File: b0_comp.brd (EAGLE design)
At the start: 93 x 70 mm, 287 parts, among them IC1 КР1006ВИ1(NE555), IC3 LM358D, IC4 78L09F, IC5 XL6009S, IC6 MEGA8-AI, IC7 74121N, IC8 4030N, IC9 LM324D, T1P T90, -26 MicroMetals Yellow-W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

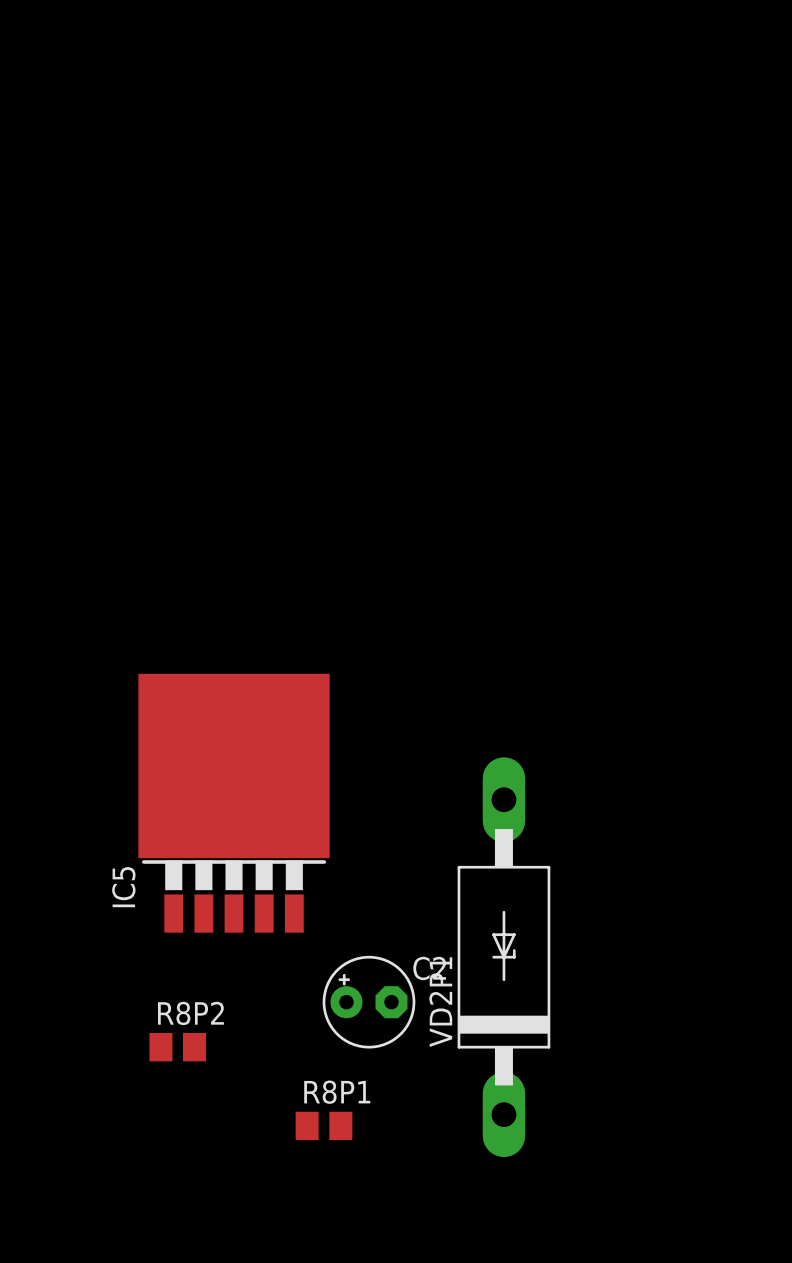
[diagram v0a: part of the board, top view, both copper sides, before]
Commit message: .
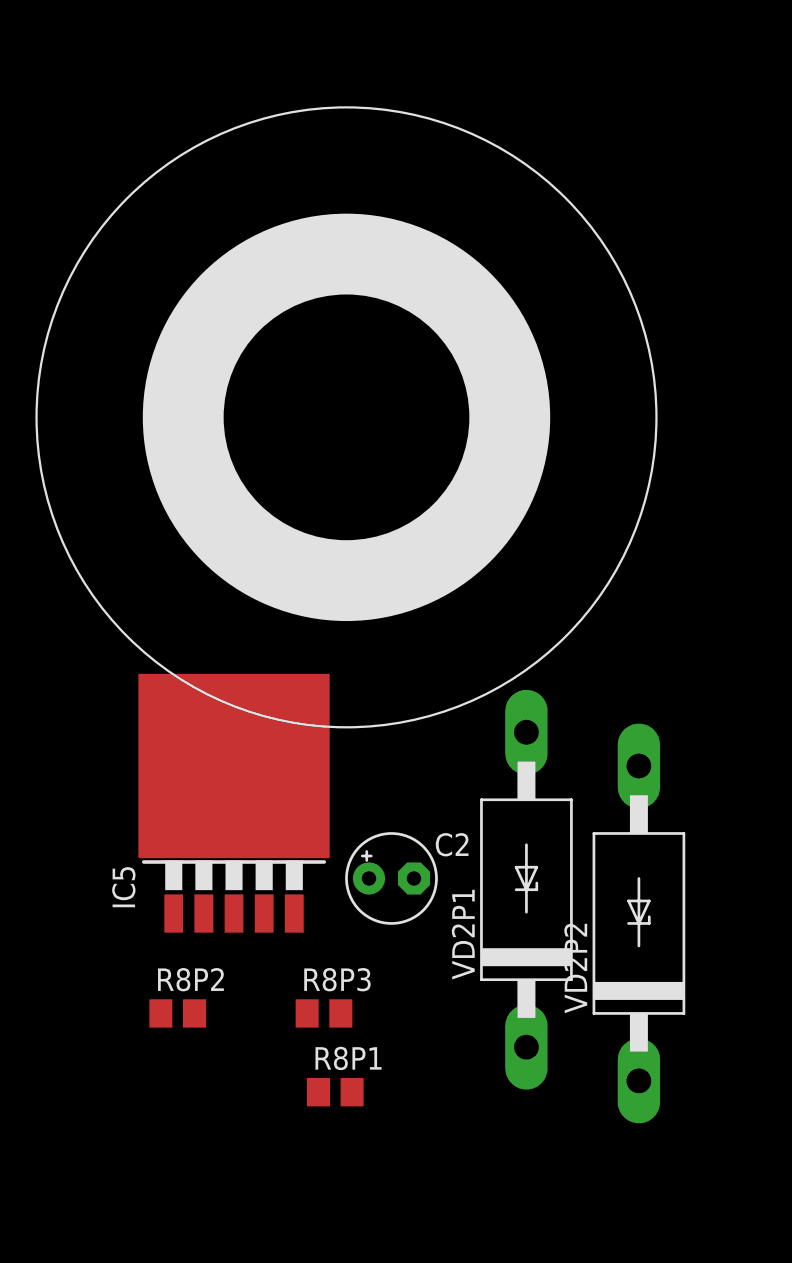
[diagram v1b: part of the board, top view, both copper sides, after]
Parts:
- added R8P3: 3k, rcl:M0805
- added T1P1: T90, -26 MicroMetals Yellow-White, b0f:R23X14
- added VD2P2: SR5200, diode:CB429-17
- C2: value (none) -> 22m
- IC5: value XL6009S -> XL6009
- moved C2 7.10 mm to (-367.7, 91.4)
- moved VD2P1 4.02 mm to (-360.0, 90.8)
- moved R8P1 2.01 mm to (-370.8, 79.4)
- moved R8P2 1.90 mm to (-379.7, 83.8)
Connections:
- new net N$190: C2.-, VD2P2.A
- new net N$191: VD2P2.C
- net N$187: now also R8P3.2; no longer R8P1.2
- net N$188: no longer C2.-
- net N$189: now also R8P3.1; no longer R8P1.1
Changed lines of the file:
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@@
 <element name="R22" library="rcl" package="M0805" value="27" x="-275.59" y="114.3" rot="MR180"/>
 <element name="R23" library="rcl" package="M0805" value="27" x="-276.225" y="123.19" rot="MR180"/>
-<element name="IC5" library="XL6009" package="TO263-5" value="XL6009S" x="-376.555" y="95.25"/>
-<element name="VD2P1" library="diode" package="CB429-17" value="SR5200" x="-361.315" y="86.995" rot="R90"/>
-<element name="C2" library="rcl" package="E2,5-5" value="" x="-368.935" y="84.455"/>
-<element name="R8P1" library="rcl" package="M0805" value="8k6" x="-371.475" y="77.47"/>
-<element name="R8P2" library="rcl" package="M0805" value="1k" x="-379.73" y="81.915"/>
+<element name="IC5" library="XL6009" package="TO263-5" value="XL6009" x="-376.555" y="95.25"/>
+<element name="VD2P1" library="diode" package="CB429-17" value="SR5200" x="-360.045" y="90.805" rot="R90"/>
+<element name="C2" library="rcl" package="E2,5-5" value="22m" x="-367.665" y="91.44"/>
+<element name="R8P1" library="rcl" package="M0805" value="8k6" x="-370.84" y="79.375"/>
+<element name="R8P2" library="rcl" package="M0805" value="1k" x="-379.73" y="83.82"/>
+<element name="R8P3" library="rcl" package="M0805" value="3k" x="-371.475" y="83.82"/>
+<element name="T1P1" library="b0f" package="R23X14" value="T90, -26 MicroMetals Yellow-White" x="-370.205" y="117.475"/>
+<element name="VD2P2" library="diode" package="CB429-17" value="SR5200" x="-353.695" y="88.9" rot="R90"/>
 </elements>
 <signals>
@@
 <wire x1="-367.0275" y1="-35.2425" x2="-364.4265" y2="-29.5275" width="0" layer="19" extent="1-1"/>
 <wire x1="-364.4265" y1="-39.0525" x2="-367.0275" y2="-35.2425" width="0" layer="19" extent="1-1"/>
-<wire x1="-380.68" y1="81.915" x2="-367.3475" y2="-3.4925" width="0" layer="19" extent="1-1"/>
-<wire x1="-379.9586" y1="89.4588" x2="-380.68" y2="81.915" width="0" layer="19" extent="1-1"/>
+<wire x1="-380.68" y1="83.82" x2="-367.3475" y2="-3.4925" width="0" layer="19" extent="1-1"/>
+<wire x1="-379.9586" y1="89.4588" x2="-380.68" y2="83.82" width="0" layer="19" extent="1-1"/>
 <wire x1="-378.2568" y1="89.4588" x2="-379.9586" y2="89.4588" width="0" layer="19" extent="1-1"/>
 </signal>
@@
 <contactref element="IC5" pad="3"/>
 <contactref element="C2" pad="+"/>
-<wire x1="-370.205" y1="84.455" x2="-376.555" y2="89.4588" width="0" layer="19" extent="1-1"/>
+<wire x1="-368.935" y1="91.44" x2="-376.555" y2="89.4588" width="0" layer="19" extent="1-1"/>
 </signal>
 <signal name="N$186">
@@
 <signal name="N$188">
 <contactref element="VD2P1" pad="A"/>
-<contactref element="C2" pad="-"/>
-<wire x1="-361.315" y1="95.885" x2="-367.665" y2="84.455" width="0" layer="19" extent="1-1"/>
 </signal>
 <signal name="N$187">
 <contactref element="VD2P1" pad="C"/>
-<contactref element="R8P1" pad="2"/>
-<wire x1="-361.315" y1="78.105" x2="-370.525" y2="77.47" width="0" layer="19" extent="1-1"/>
+<contactref element="R8P3" pad="2"/>
+<wire x1="-370.525" y1="83.82" x2="-360.045" y2="81.915" width="0" layer="19" extent="1-1"/>
 </signal>
 <signal name="N$189">
-<contactref element="R8P1" pad="1"/>
 <contactref element="R8P2" pad="2"/>
 <contactref element="IC5" pad="5"/>
-<wire x1="-372.425" y1="77.47" x2="-378.78" y2="81.915" width="0" layer="19" extent="1-1"/>
-<wire x1="-373.1514" y1="89.4588" x2="-378.78" y2="81.915" width="0" layer="19" extent="1-1"/>
+<contactref element="R8P3" pad="1"/>
+<wire x1="-373.1514" y1="89.4588" x2="-378.78" y2="83.82" width="0" layer="19" extent="1-1"/>
+<wire x1="-372.425" y1="83.82" x2="-378.78" y2="83.82" width="0" layer="19" extent="1-1"/>
+</signal>
+<signal name="N$190">
+<contactref element="C2" pad="-"/>
+<contactref element="VD2P2" pad="A"/>
+<wire x1="-353.695" y1="97.79" x2="-366.395" y2="91.44" width="0" layer="19" extent="1-1"/>
+</signal>
+<signal name="N$191">
+<contactref element="VD2P2" pad="C"/>
 </signal>
 </signals>
